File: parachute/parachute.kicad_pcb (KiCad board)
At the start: 2 copper layers, 16 parts, among them J1 servo, J2 power, J3 hmi, J5 trigger_rpi, J6 trigger_lauch, U1 LTV-814, U3 RP2040, U4 LTV-814

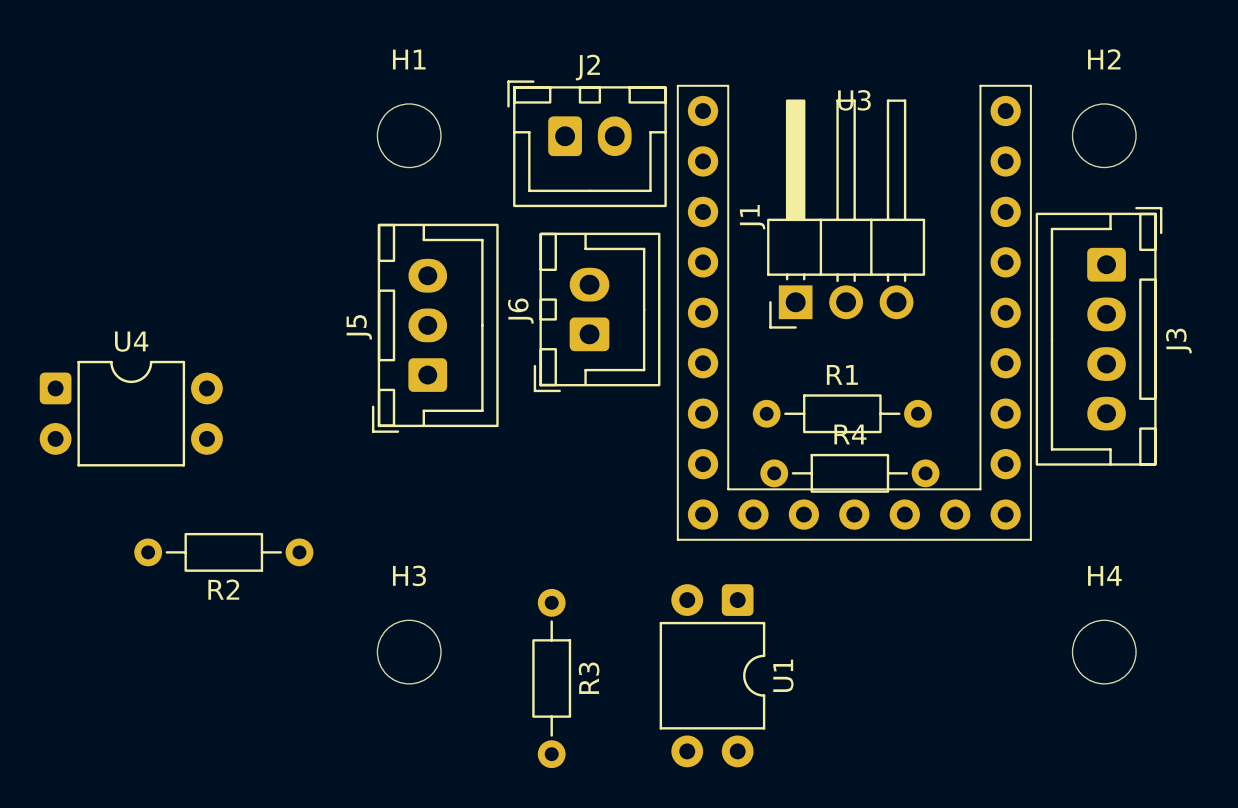
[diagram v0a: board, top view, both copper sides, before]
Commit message: agencement et piste cuivre pour PCB parachute
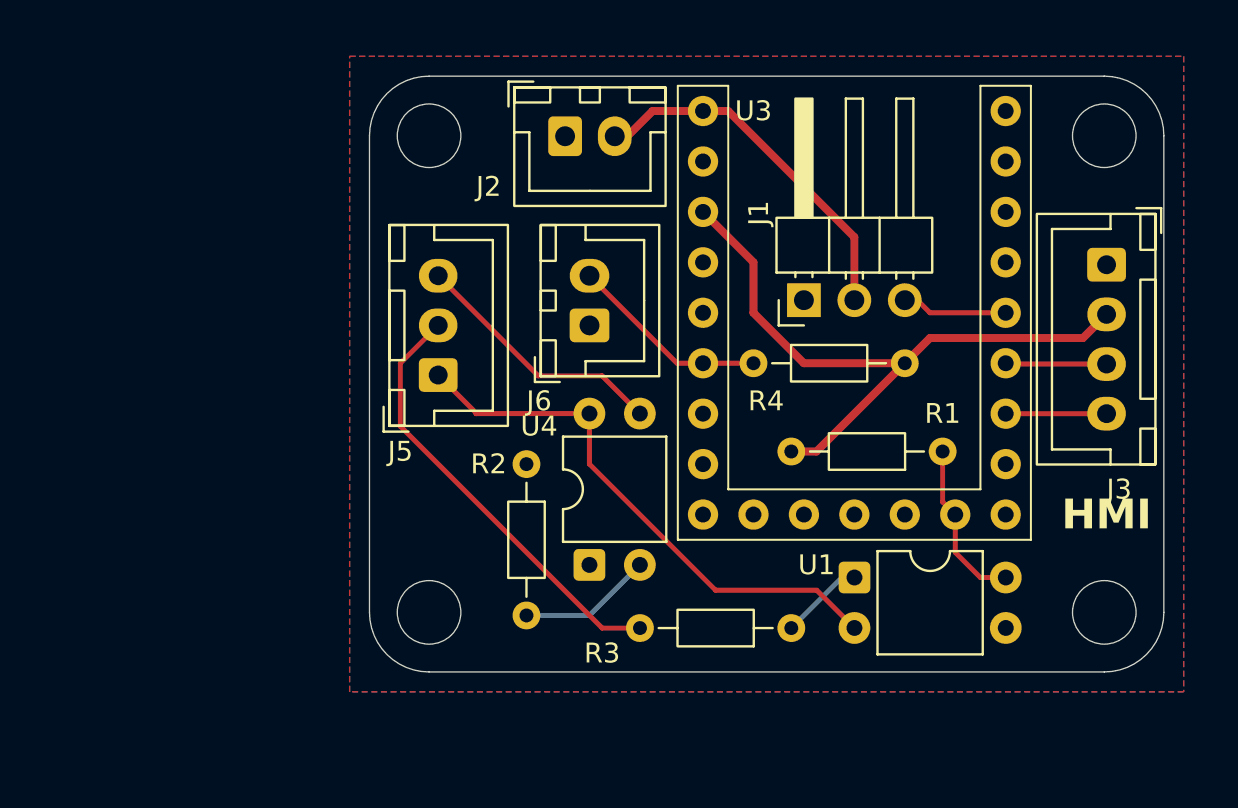
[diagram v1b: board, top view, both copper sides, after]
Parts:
- moved U4 28.3 mm to (132.1, 94.6), turned to 90 degrees
- moved R2 12.3 mm to (128.9, 89.5), turned to -90 degrees
- moved R3 12.1 mm to (142.2, 97.8), turned to 180 degrees
- moved R1 9.06 mm to (149.9, 88.9), turned to 180 degrees
- moved U1 5.99 mm to (145.4, 95.2), turned to 0 degrees
- moved R4 5.64 mm to (140.3, 84.5)
- moved H3 2.24 mm to (124.0, 97.0)
- moved H4 2.00 mm to (158.0, 97.0)
- moved H1 1.00 mm to (124.0, 73.0)
- moved J5 0.52 mm to (124.5, 85.0)
- moved J6 0.45 mm to (132.1, 82.5)
- moved J1 0.43 mm to (142.9, 81.3)
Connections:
- U3 pad 14: unconnected-(U3-GPIO14-Pad14) -> /TRIGGER
- U3 pad 17: unconnected-(U3-GPIO14-Pad17) -> /LED_TIMER_TRIGGED
- U3 pad 18: unconnected-(U3-GPIO14-Pad18) -> /LED_OPEN
- U3 pad 19: unconnected-(U3-GPIO14-Pad19) -> /SERVO
- U3 pad 4: /LED_OPEN -> unconnected-(U3-GPIO29-Pad4)
- U3 pad 5: /LED_TIMER_TRIGGED -> unconnected-(U3-GPIO28-Pad5)
- U3 pad 7: /TRIGGER -> unconnected-(U3-GPIO26-Pad7)
- U3 pad 8: /SERVO -> /parachute_open
- U3 pad 9: /parachute_open -> unconnected-(U3-GPIO14-Pad9)
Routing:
- net +3V3: track 0.00 -> 33.5 mm
- net Net-(J5-Pin_1): track 0.00 -> 27.8 mm
- net Net-(J5-Pin_2): track 0.00 -> 22.1 mm
- net +5V: track 0.00 -> 18.4 mm
- net Net-(J5-Pin_3): track 0.00 -> 13.0 mm
- net /BUTTON_LAUCHED: track 0.00 -> 10.1 mm
- net /TRIGGER: track 0.00 -> 8.41 mm
- net Net-(R2-Pad2): track 0.00 -> 6.76 mm
- net /SERVO: track 0.00 -> 5.34 mm
- net /LED_OPEN: track 0.00 -> 5.10 mm
- net /LED_TIMER_TRIGGED: track 0.00 -> 5.08 mm
- net Net-(R3-Pad1): track 0.00 -> 4.23 mm
- added copper zone on B.Cu, net GND
- added copper zone on F.Cu, net GND
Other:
- board outline added: 40 x 30 mm
- board text added: "10k"
- board text added: "330"
- board text added: "5V"
- board text added: "CONTROL"
- board text added: "HMI"
- board text added: "LAUCH"
- board text added: "SERVO"
